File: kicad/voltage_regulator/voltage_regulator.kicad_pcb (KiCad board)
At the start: 2 copper layers, 135.9 x 78.7 mm, 18 parts

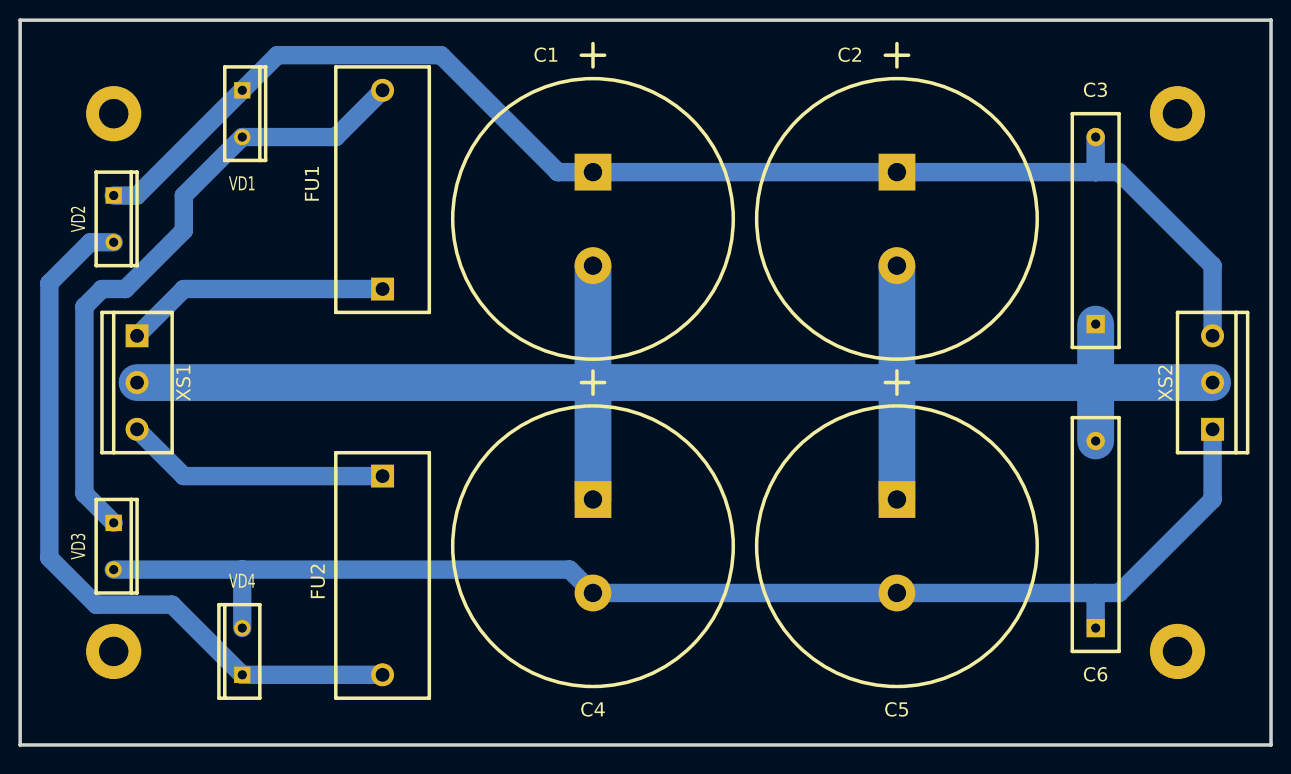
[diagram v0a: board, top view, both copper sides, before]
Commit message: New commit.
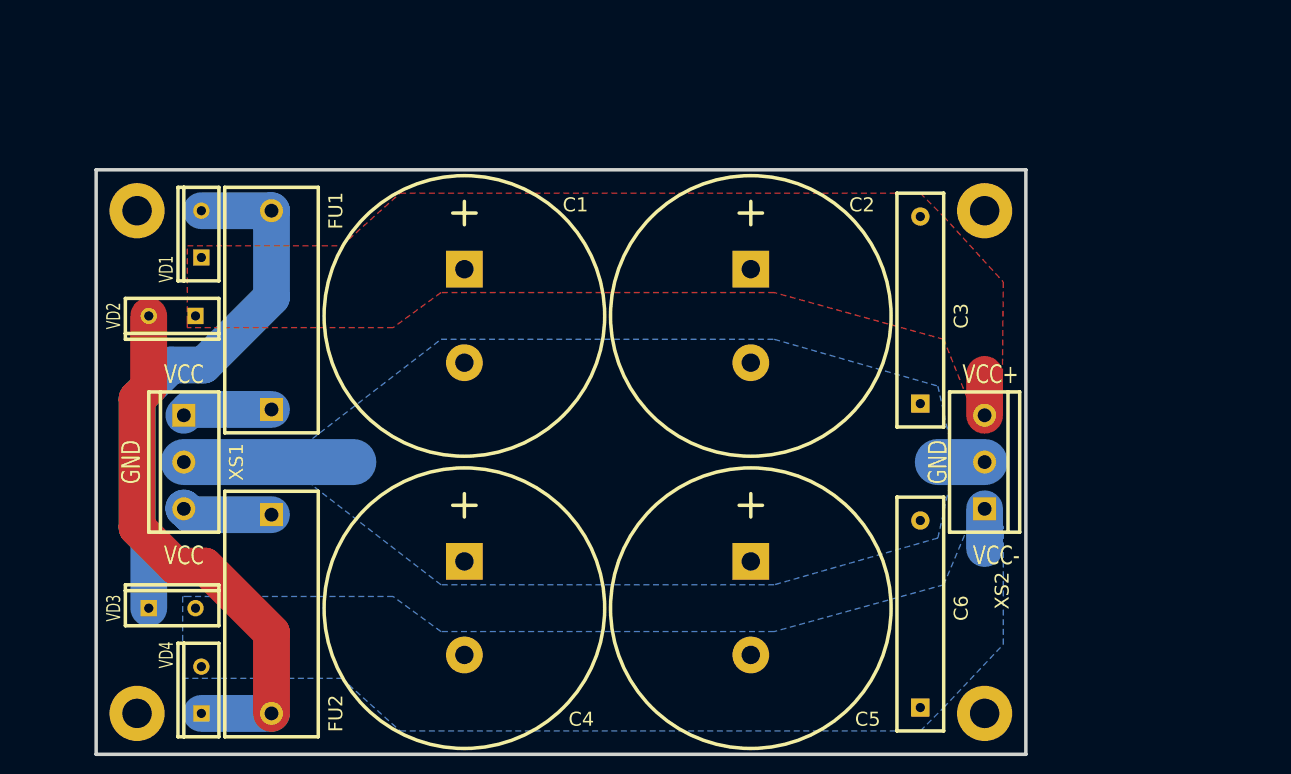
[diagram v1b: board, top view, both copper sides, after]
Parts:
- moved XS2 26.2 mm to (178.4, 96.3)
- moved C6 20.9 mm to (171.4, 122.9)
- moved C3 20.9 mm to (171.4, 89.9)
- moved C2 19.1 mm to (153.0, 80.4)
- moved 1_PIN 18.6 mm to (182.9, 65.8)
- moved FU1 17.8 mm to (101.0, 85.5)
- moved 1_PIN 17.6 mm to (182.9, 122.9)
- moved C1 17.5 mm to (121.9, 80.4)
- moved C5 17.2 mm to (153.0, 112.1)
- moved C4 15.5 mm to (121.9, 112.1)
- moved VD1 13.8 mm to (93.3, 71.5), turned to 180 degrees
- moved FU2 12.8 mm to (101.0, 107.1)
- moved VD2 12.3 mm to (90.2, 80.4), turned to 270 degrees
- moved 1_PIN 11.0 mm to (76.2, 124.8)
- moved XS1 10.0 mm to (91.4, 96.3)
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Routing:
- net /GND: track 180.3 -> 23.5 mm
- net /VCC+: track 146.6 -> 4.45 mm
- net /VCC-: track 142.4 -> 4.32 mm
- net N-000004: track 80.1 -> 59.2 mm
- net N-000006: track 28.8 -> 9.79 mm
- net N-000005: track 28.8 -> 9.90 mm
- net N-000003: track 69.2 -> 59.5 mm
- added copper zone on B.Cu, net /GND
- added copper zone on F.Cu, net /VCC+
- added copper zone on B.Cu, net /VCC-
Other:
- board size 135.9 x 78.7 mm -> 101 x 63.5 mm
- net class Default: clearance 1.00076 -> 0.5; trace_width 0.50038 -> 1
- rule trace_clearance: 1.00076 -> 0.5
- board text added: "GND"
- board text added: "VCC"
- board text added: "VCC+"
- board text added: "VCC-"
